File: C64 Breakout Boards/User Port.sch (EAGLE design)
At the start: 2 parts, among them CN1 USERPORT-C64-EDGE, X1 87758-2416

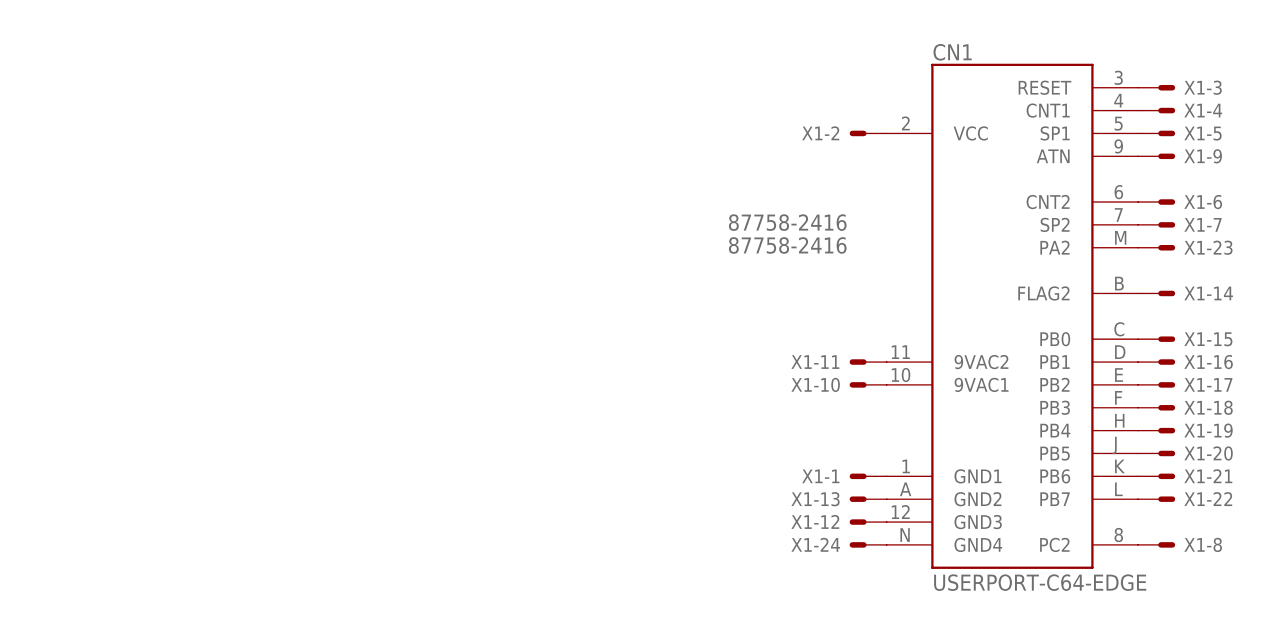
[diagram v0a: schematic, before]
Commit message: Breakout Boards done
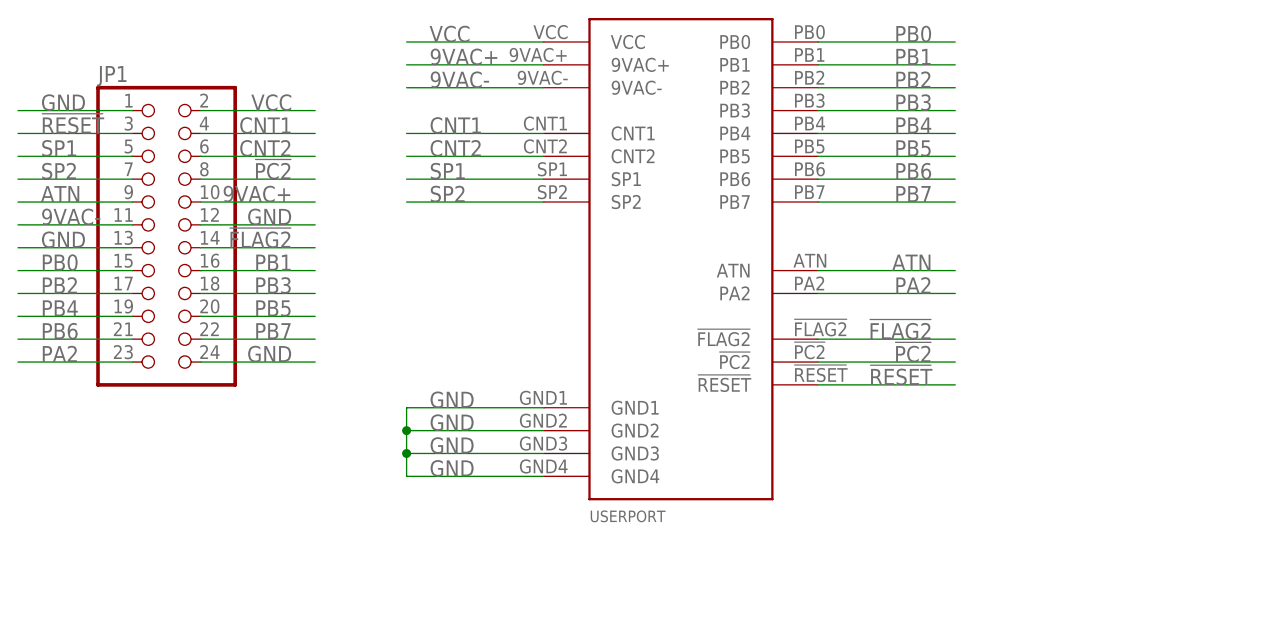
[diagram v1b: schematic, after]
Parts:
- removed CN1: USERPORT-C64-EDGE, 0RB_Commodore:USERPORT-C64-EDGE
- removed X1: 87758-2416, con-molex:87758-2416
- added JP1: (no value), pinhead:PINHD-2X12
- added USERPORT: C64_USER, 0myparts:C64_USER
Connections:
- removed net N$1: CN1.GND1, X1-1.S
- removed net N$10: CN1.9VAC1, X1-10.S
- removed net N$11: CN1.9VAC2, X1-11.S
- removed net N$12: CN1.GND3, X1-12.S
- removed net N$13: CN1.GND2, X1-13.S
- removed net N$14: CN1.FLAG2, X1-14.S
- removed net N$15: CN1.PB0, X1-15.S
- removed net N$16: CN1.PB1, X1-16.S
- removed net N$17: CN1.PB2, X1-17.S
- removed net N$18: CN1.PB3, X1-18.S
- removed net N$19: CN1.PB4, X1-19.S
- removed net N$2: CN1.VCC, X1-2.S
- removed net N$20: CN1.PB5, X1-20.S
- removed net N$21: CN1.PB6, X1-21.S
- removed net N$22: CN1.PB7, X1-22.S
- removed net N$23: CN1.PA2, X1-23.S
- removed net N$24: CN1.GND4, X1-24.S
- removed net N$3: CN1.RESET, X1-3.S
- removed net N$4: CN1.CNT1, X1-4.S
- removed net N$5: CN1.SP1, X1-5.S
- removed net N$6: CN1.CNT2, X1-6.S
- removed net N$7: CN1.SP2, X1-7.S
- removed net N$8: CN1.PC2, X1-8.S
- removed net N$9: CN1.ATN, X1-9.S
- new net !FLAG2: JP1.14, USERPORT.!FLAG2
- new net !PC2: JP1.8, USERPORT.!PC2
- new net !RESET: JP1.3, USERPORT.!RESET
- new net 9VAC+: JP1.10, USERPORT.9VAC+
- new net 9VAC-: JP1.11, USERPORT.9VAC-
- new net ATN: JP1.9, USERPORT.ATN
- new net CNT1: JP1.4, USERPORT.CNT1
- new net CNT2: JP1.6, USERPORT.CNT2
- new net GND: JP1.1, JP1.12, JP1.13, JP1.24, USERPORT.GND1, USERPORT.GND2, USERPORT.GND3, USERPORT.GND4
- new net PA2: JP1.23, USERPORT.PA2
- new net PB0: JP1.15, USERPORT.PB0
- new net PB1: JP1.16, USERPORT.PB1
- new net PB2: JP1.17, USERPORT.PB2
- new net PB3: JP1.18, USERPORT.PB3
- new net PB4: JP1.19, USERPORT.PB4
- new net PB5: JP1.20, USERPORT.PB5
- new net PB6: JP1.21, USERPORT.PB6
- new net PB7: JP1.22, USERPORT.PB7
- new net SP1: JP1.5, USERPORT.SP1
- new net SP2: JP1.7, USERPORT.SP2
- new net VCC: JP1.2, USERPORT.VCC
